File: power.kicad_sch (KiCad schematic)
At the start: 40 parts, among them U11 NCP186BMX185TAG, U3 STM32H745ZIT6, U4 NCP186AMX390TAG, U5 NCP186BMX185TAG

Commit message: New structure for holding parts, symbols, and footprints
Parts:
- FL2: footprint BLM18EG221SN1D:BEADC1608X95N -> CivicAlert:FCM1608KF-601T03
- PWR1: footprint LTST-C170KRKT:LED_LTST-C170KRKT_LTO -> CivicAlert:LTST-C170KRKT
- U11, U5: footprint NCP186BMX185TAG:XDFN8_1P7X1P3_ONS -> CivicAlert:NCP186BMX185TAG
- U3: footprint STM32H745ZIT6:LQFP-144 -> CivicAlert:STM32H745ZIT6
- U4: footprint NCP186AMX390TAG:XDFN8_1P7X1P3_ONS -> CivicAlert:NCP186AMX390TAG
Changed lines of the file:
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@@
 			)
 		)
-		(property "Footprint" "NCP186AMX390TAG:XDFN8_1P7X1P3_ONS"
+		(property "Footprint" "CivicAlert:NCP186AMX390TAG"
 			(at 105.41 170.18 0)
 			(effects
@@
 			)
 		)
-		(property "Footprint" "NCP186BMX185TAG:XDFN8_1P7X1P3_ONS"
+		(property "Footprint" "CivicAlert:NCP186BMX185TAG"
 			(at 105.41 123.19 0)
 			(effects
@@
 			)
 		)
-		(property "Footprint" "NCP186BMX185TAG:XDFN8_1P7X1P3_ONS"
+		(property "Footprint" "CivicAlert:NCP186BMX185TAG"
 			(at 227.33 139.7 0)
 			(effects
@@
 			)
 		)
-		(property "Footprint" "LTST-C170KRKT:LED_LTST-C170KRKT_LTO"
+		(property "Footprint" "CivicAlert:LTST-C170KRKT"
 			(at 54.61 54.61 0)
 			(effects
@@
 			)
 		)
-		(property "Footprint" "BLM18EG221SN1D:BEADC1608X95N"
+		(property "Footprint" "CivicAlert:FCM1608KF-601T03"
 			(at 146.05 81.28 0)
 			(effects
@@
 			)
 		)
-		(property "Footprint" "STM32H745ZIT6:LQFP-144"
+		(property "Footprint" "CivicAlert:STM32H745ZIT6"
 			(at 194.31 26.67 0)
 			(effects

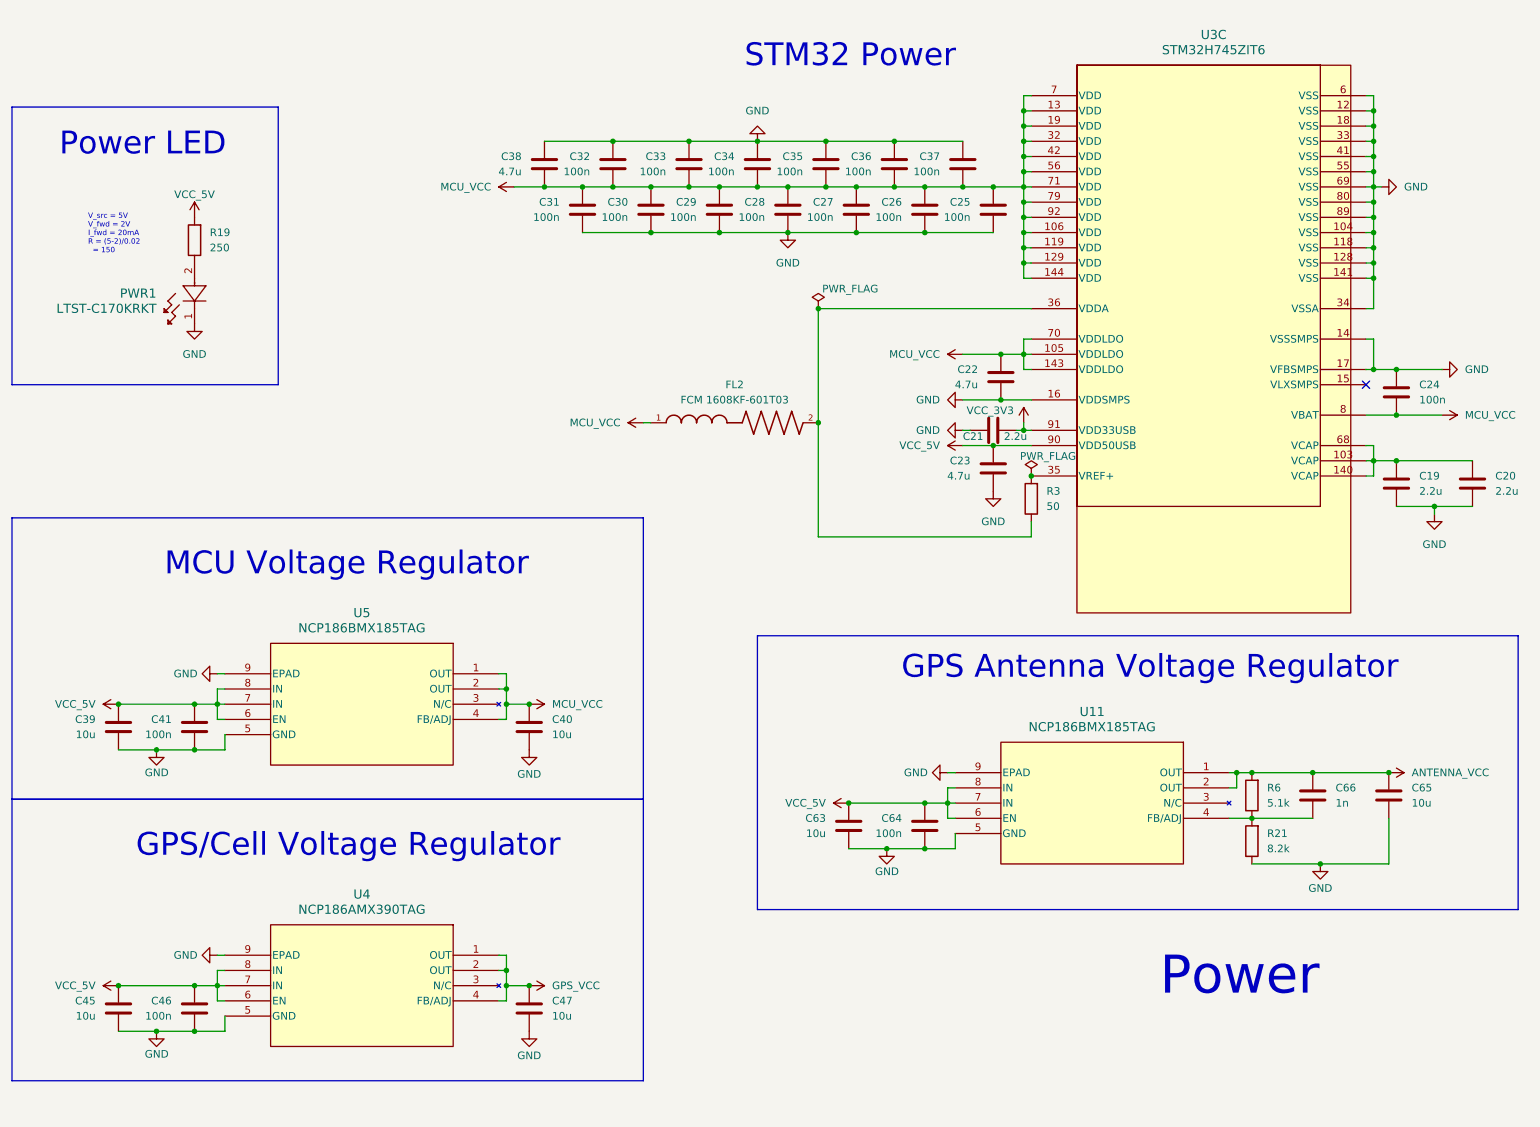
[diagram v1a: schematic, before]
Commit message: Update for RevB
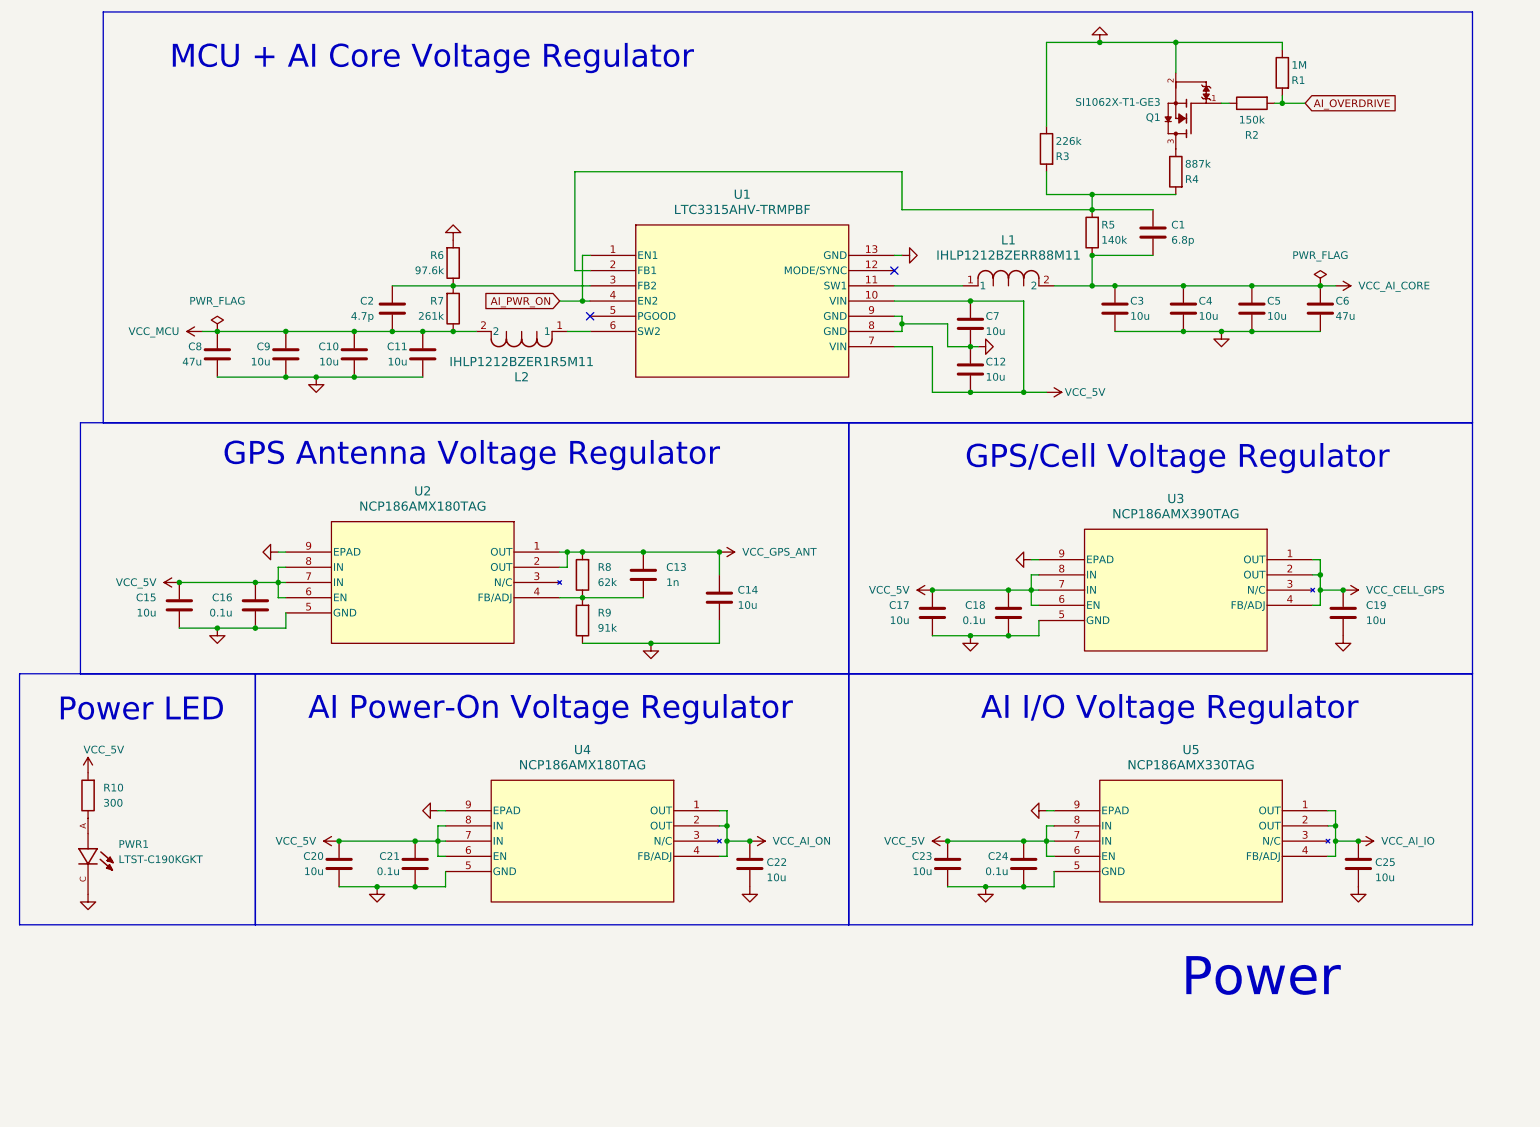
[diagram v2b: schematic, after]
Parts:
- removed C26, C27, C28, C29, C30, C31, C32, C33, C34, C35, C36, C37, C41, C46, C64: 100n, Capacitor_SMD:C_0402_1005Metric, symbol Device:C
- removed C38: 4.7u, Capacitor_SMD:C_0402_1005Metric, symbol Device:C
- removed C39, C40, C45, C47, C63, C65: 10u, Capacitor_SMD:C_0402_1005Metric, symbol Device:C
- removed C66: 1n, Capacitor_SMD:C_0402_1005Metric, symbol Device:C
- removed FL2: FCM 1608KF-601T03, CivicAlert:FCM1608KF-601T03, symbol FCM1608KF-601T03:BLM18EG221SN1D
- removed PWR1: LTST-C170KRKT, CivicAlert:LTST-C170KRKT, symbol LTST-C170KRKT:LTST-C170KRKT
- removed R19: 250, Resistor_SMD:R_0402_1005Metric, symbol Device:R
- removed R21: 8.2k, Resistor_SMD:R_0402_1005Metric, symbol Device:R
- removed U11, U5: NCP186BMX185TAG, CivicAlert:NCP186BMX185TAG, symbol NCP186BMX185TAG:NCP186BMX185TAG
- removed U3: STM32H745ZIT6, CivicAlert:STM32H745ZIT6, symbol STM32H745ZIT6:STM32H745ZIT6
- removed U4: NCP186AMX390TAG, CivicAlert:NCP186AMX390TAG, symbol NCP186AMX390TAG:NCP186AMX390TAG
- added C1: 6.8p, Capacitor_SMD:C_0402_1005Metric, symbol Device:C
- added C10, C11, C12, C3, C4, C5, C7, C9: 10u, Capacitor_SMD:C_0805_2012Metric, symbol Device:C
- added C13: 1n, Capacitor_SMD:C_0402_1005Metric, symbol Device:C
- added C14, C15, C17: 10u, Capacitor_SMD:C_0603_1608Metric, symbol Device:C
- added C16, C18: 0.1u, Capacitor_SMD:C_0402_1005Metric, symbol Device:C
- added C2: 4.7p, Capacitor_SMD:C_0402_1005Metric, symbol Device:C
- added C6, C8: 47u, Capacitor_SMD:C_1206_3216Metric, symbol Device:C
- added L1: IHLP1212BZERR88M11, CivicAlert:IHLP1212BZERR88M11, symbol IHLP1212BZERR88M11:IHLP1212BZERR88M11
- added L2: IHLP1212BZER1R5M11, CivicAlert:IHLP1212BZER1R5M11, symbol IHLP1212BZER1R5M11:IHLP1212BZER1R5M11
- added PWR1: LTST-C190KGKT, CivicAlert:LTST-C190KGKT, symbol LTST-C190KGKT:LTST-C190KGKT
- added Q1: SI1062X-T1-GE3, CivicAlert:SI1062X-T1-GE3, symbol SI1062X-T1-GE3:SI1062X-T1-GE3
- added R1: 1M, Resistor_SMD:R_0402_1005Metric, symbol Device:R
- added R10: 300, Resistor_SMD:R_0402_1005Metric, symbol Device:R
- added R2: 150k, Resistor_SMD:R_0402_1005Metric, symbol Device:R
- added R4: 887k, Resistor_SMD:R_0603_1608Metric, symbol Device:R
- added R5: 140k, Resistor_SMD:R_0603_1608Metric, symbol Device:R
- added R7: 261k, Resistor_SMD:R_0603_1608Metric, symbol Device:R
- added R8: 62k, Resistor_SMD:R_0402_1005Metric, symbol Device:R
- added R9: 91k, Resistor_SMD:R_0402_1005Metric, symbol Device:R
- added U1: LTC3315AHV-TRMPBF, CivicAlert:LTC3315AHV, symbol LTC3315AHV:LTC3315AHV-TRMPBF
- added U2, U4: NCP186AMX180TAG, CivicAlert:NCP186AMX, symbol NCP186AMX180TAG:NCP186AMX180TAG
- added U3: NCP186AMX390TAG, CivicAlert:NCP186AMX, symbol NCP186AMX390TAG:NCP186AMX390TAG
- added U5: NCP186AMX330TAG, CivicAlert:NCP186AMX, symbol NCP186AMX330TAG:NCP186AMX330TAG
- C19, C20: value 2.2u -> 10u; footprint Capacitor_SMD:C_0402_1005Metric -> Capacitor_SMD:C_0603_1608Metric; MANUFACTURER Murata -> (none); MPN GRT155C71A225KE13D -> (none); Manufacturer (none) -> Murata
- C21: value 2.2u -> 0.1u; MANUFACTURER Murata -> (none); MPN GRT155C71A225KE13D -> (none); Manufacturer (none) -> Murata
- C22, C23: value 4.7u -> 10u; footprint Capacitor_SMD:C_0402_1005Metric -> Capacitor_SMD:C_0603_1608Metric; MANUFACTURER Murata -> (none); MPN GRT155D70J475ME13D -> (none); Manufacturer (none) -> Murata
- C24: value 100n -> 0.1u; MANUFACTURER Murata -> (none); MPN GRT155R71H104KE01D -> (none); Manufacturer (none) -> Murata
- C25: value 100n -> 10u; footprint Capacitor_SMD:C_0402_1005Metric -> Capacitor_SMD:C_0603_1608Metric; MANUFACTURER Murata -> (none); MPN GRT155R71H104KE01D -> (none); Manufacturer (none) -> Murata
- R3: value 50 -> 226k; footprint Resistor_SMD:R_0402_1005Metric -> Resistor_SMD:R_0603_1608Metric; Manufacturer (none) -> Yageo
- R6: value 5.1k -> 97.6k; footprint Resistor_SMD:R_0402_1005Metric -> Resistor_SMD:R_0603_1608Metric; Manufacturer (none) -> Yageo
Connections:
- net ANTENNA_VCC is gone; now on net GND: R6.2
- net VCC_3V3 is gone; now on net VCC_5V: C21.1
- net GND: now also C24.2, R3.1, C10.2, C11.2, C12.1, C14.2, C15.2, C16.2, C17.2, C18.2, C3.2, C4.2, C5.2, C6.2, C7.2, C8.2, C9.2, PWR1.C, Q1.2, R1.1, R9.1, U1.13 (GND), U1.8 (GND), U1.9 (GND), U2.5 (GND), U2.9 (EPAD), U3.5 (GND), U3.9 (EPAD), U4.5 (GND), U4.9 (EPAD), U5.5 (GND), U5.9 (EPAD); no longer C24.1
- net VCC_5V: now also C20.1, C24.1, C12.2, C15.1, C16.1, C17.1, C18.1, C7.1, R10.2, U1.10 (VIN), U1.7 (VIN), U2.6 (EN), U2.7 (IN), U2.8 (IN), U3.6 (EN), U3.7 (IN), U3.8 (IN), U4.6 (EN), U4.7 (IN), U4.8 (IN), U5.6 (EN), U5.7 (IN), U5.8 (IN)
- net VCC_CELL_GPS: now reaches C19.1
- net VCC_CELL_GPS: now also U3.1 (OUT), U3.2 (OUT), U3.4 (FB/ADJ); no longer C20.1
- net at R6.1: now also C2.1, R7.2, U1.3 (FB2)
- net at R3.2: now also C1.1, R4.2, R5.2, U1.2 (FB1)
- removed net MCU_VCC: C22.1, C24.2, C25.1
- new net: Q1.1, R2.1
- new net: Q1.3, R4.1
- new net: C13.2, R8.1, R9.2, U2.4 (FB/ADJ)
- new net: L2.1, U1.6 (SW2)
- new net: PWR1.A, R10.1
- new net: L1.1, U1.11 (SW1)
- new net AI_OVERDRIVE: R1.2, R2.2
- new net AI_PWR_ON: U1.1 (EN1), U1.4 (EN2)
- new net VCC_AI_CORE: C1.2, C3.1, C4.1, C5.1, C6.1, L1.2, R5.1
- new net VCC_AI_IO: C25.1, U5.1 (OUT), U5.2 (OUT), U5.4 (FB/ADJ)
- new net VCC_AI_ON: C22.1, U4.1 (OUT), U4.2 (OUT), U4.4 (FB/ADJ)
- new net VCC_GPS_ANT: C13.1, C14.1, R8.2, U2.1 (OUT), U2.2 (OUT)
- new net VCC_MCU: C10.1, C11.1, C2.2, C8.1, C9.1, L2.2, R7.1
- no-connect marks 1 -> 2
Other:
- note added: "AI I/O Voltage Regulator"
- note added: "AI Power-On Voltage Regulator"
- note added: "MCU + AI Core Voltage Regulator"
- note removed: "MCU Voltage Regulator"
- note removed: "STM32 Power"
- note removed: "V_src = 5V V_fwd = 2V I_fwd = 20mA R = (5-2)/0.02 = 150"

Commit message: Finalize RevB
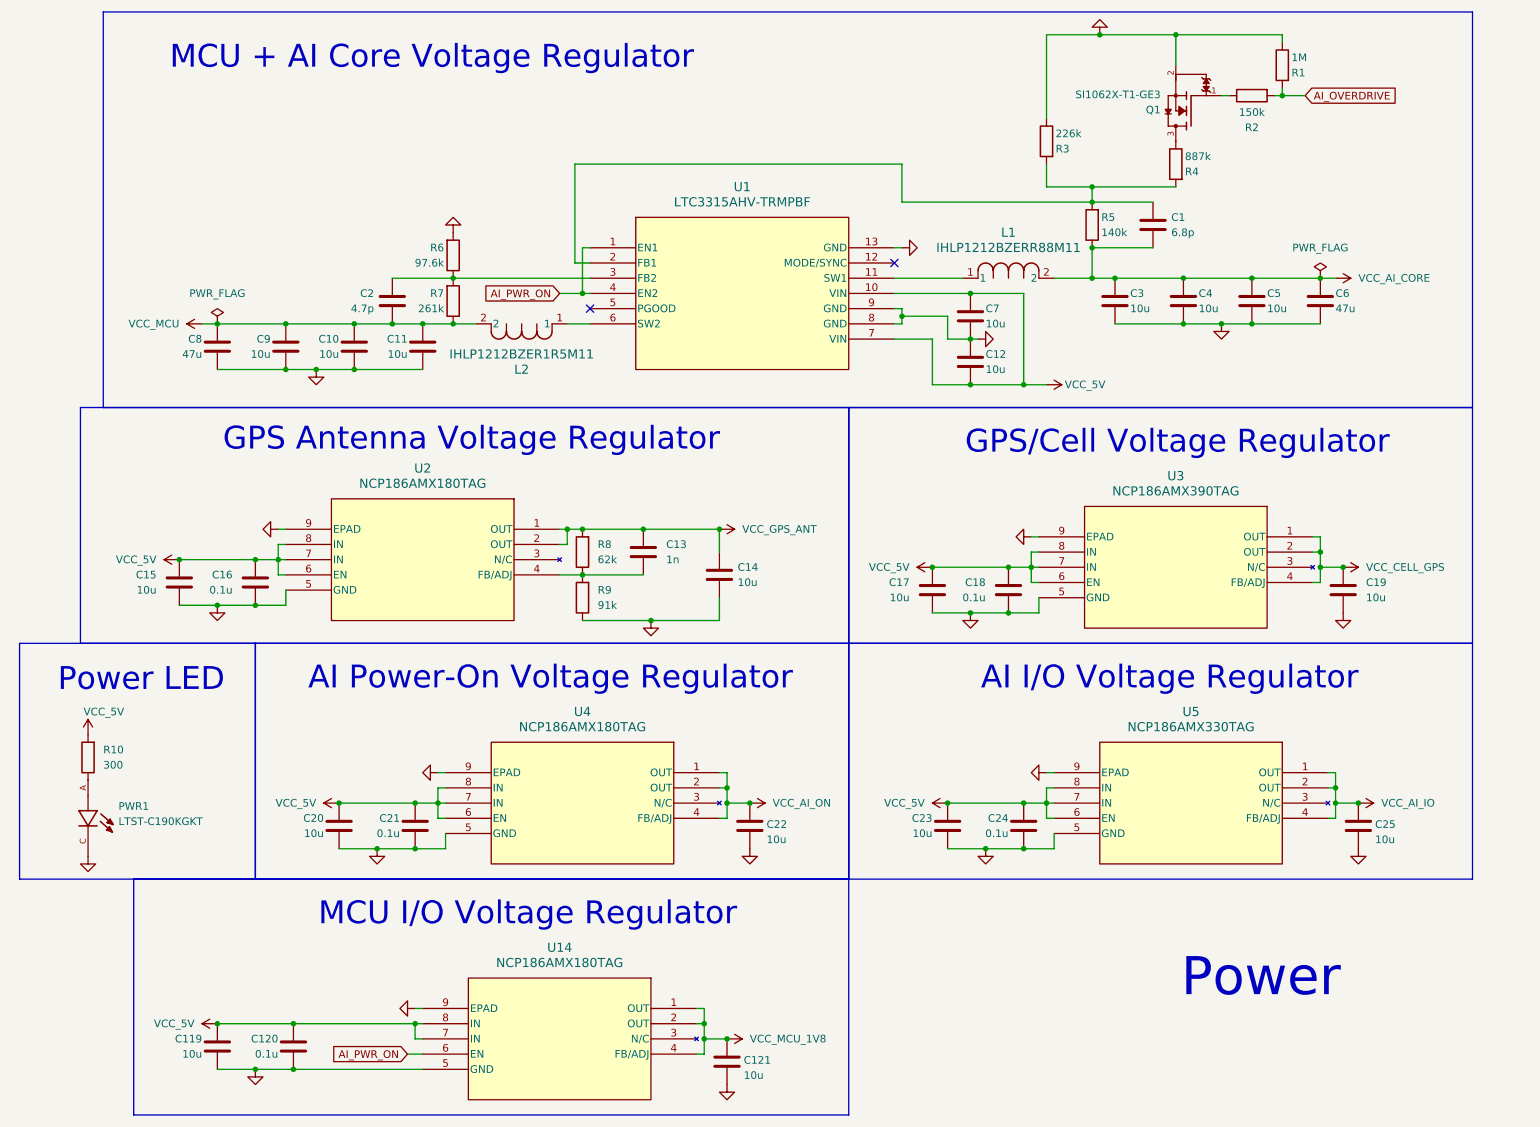
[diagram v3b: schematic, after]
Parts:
- added C119, C121: 10u, Capacitor_SMD:C_0603_1608Metric, symbol Device:C
- added C120: 0.1u, Capacitor_SMD:C_0402_1005Metric, symbol Device:C
- added U14: NCP186AMX180TAG, CivicAlert:NCP186AMX, symbol NCP186AMX180TAG:NCP186AMX180TAG
- C1: MPN (none) -> GCM1555C1H6R8BA16J
- C10, C11, C12, C3, C4, C5, C7, C9: MPN (none) -> CGA4J1X7R0J106M125AC
- C13: MPN (none) -> GRM155R71H102JA01J
- C14, C15, C17, C19, C20, C22, C23, C25: MPN (none) -> GRM188Z71A106KA73D
- C16, C18, C21, C24: MPN (none) -> GRM155R71C104KA88J
- C2: MPN (none) -> GCM1555C1H4R7CA16D
- C6, C8: MPN (none) -> C3216X7S0J476M160AC
- L1: MPN (none) -> IHLP1212BZERR88M11
- L2: MPN (none) -> IHLP1212BZER1R5M11
- PWR1: MPN (none) -> LTST-C190KGKT
- Q1: MPN (none) -> SI1062X-T1-GE3
- R3: MPN (none) -> RT0603BRD07226KL
- R4: MPN (none) -> RT0603BRD07887KL
- R5: MPN (none) -> RT0603BRD07140KL
- R6: MPN (none) -> RT0603BRD0797K6L
- R7: MPN (none) -> RT0603BRD07261KL
- U1: MPN (none) -> LTC3315AHV-TRMPBF
- U2, U4: MPN (none) -> NCP186AMX180TAG
- U3: MPN (none) -> NCP186AMX390TAG
- U5: MPN (none) -> NCP186AMX330TAG
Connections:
- net AI_PWR_ON: now also U14.6 (EN)
- net GND: now also C119.2, C120.2, C121.2, U14.5 (GND), U14.9 (EPAD)
- net VCC_5V: now also C119.1, C120.1, U14.7 (IN), U14.8 (IN)
- new net VCC_MCU_1V8: C121.1, U14.1 (OUT), U14.2 (OUT), U14.4 (FB/ADJ)
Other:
- note added: "MCU I/O Voltage Regulator"
- moved on the sheet: C1, C10, C11, C12, C13, C14, C15, C16, C17, C18, C19, C2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
